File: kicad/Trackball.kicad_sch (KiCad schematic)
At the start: 38 parts, among them J1 Conn_01x04, J101 Conn_02x03_Counter_Clockwise, SW1 Push_Button, SW101 Push_Button, SW102 Push_Button, SW103 Push_Button, SW104 Push_Button, SW106 Push_Button, SW2 Push_Button, SW3 RotaryEncoder_Switch_MP, U103 TCR2EF19, U2 PMW3360, U4 TLV73333PDBV, U7 ESP32-S3-WROOM-2

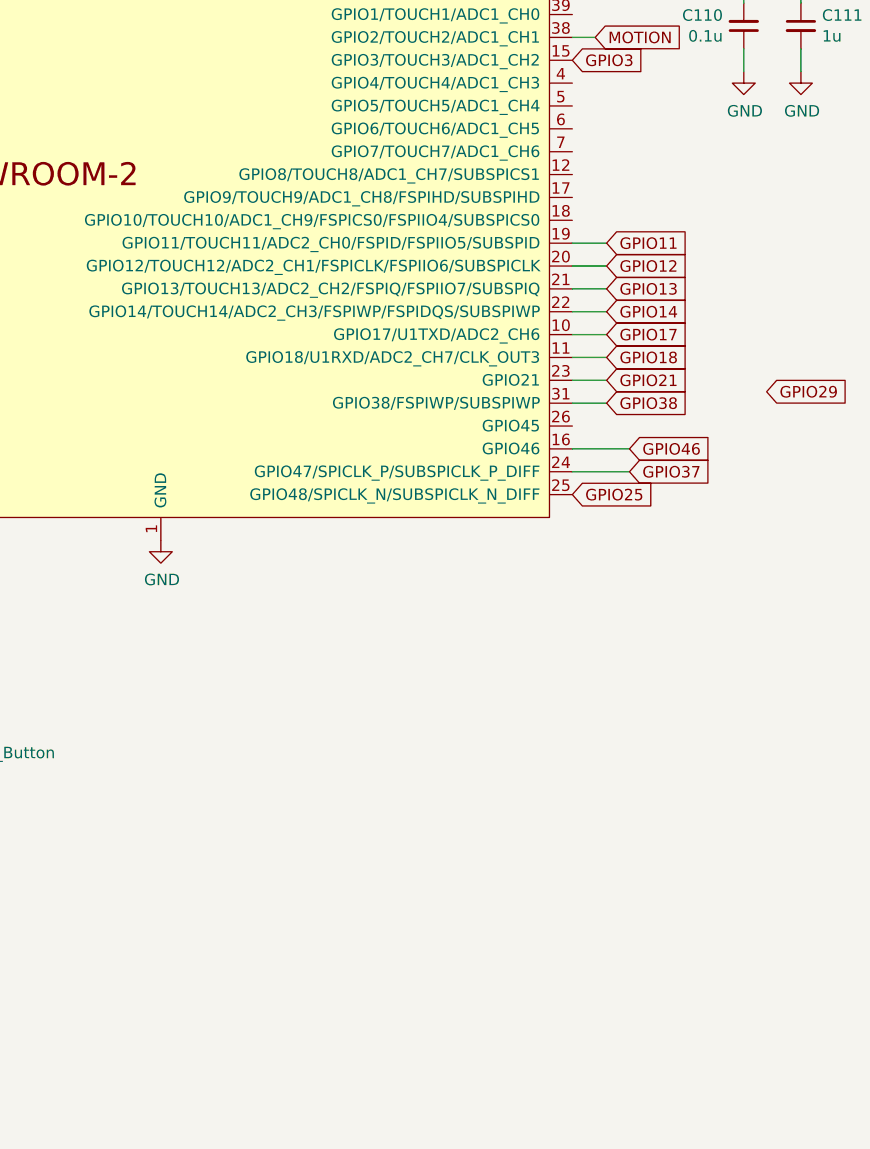
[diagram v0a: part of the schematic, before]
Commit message: V1 prebuild
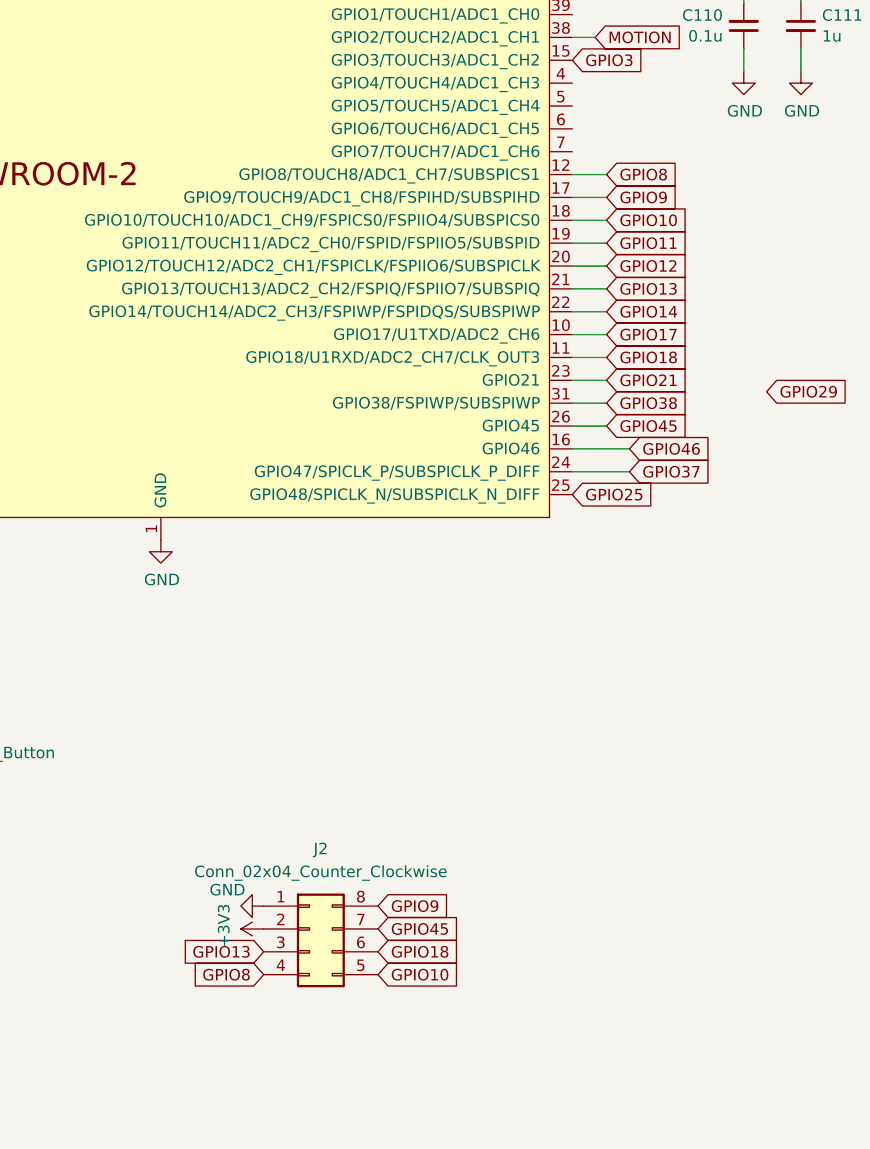
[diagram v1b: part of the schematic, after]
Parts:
- added J2: Conn_02x04_Counter_Clockwise, Connector_IDC:IDC-Header_2x04_P2.54mm_Vertical, symbol Connector_Generic:Conn_02x04_Counter_Clockwise
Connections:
- net +3V3: now also J2.2 (Pin_2)
- net GND: now also J2.1 (Pin_1)
- net GPIO13: now also J2.3 (Pin_3)
- net GPIO18: now also J2.6 (Pin_6)
- net GPIO8: now reaches U7.12 (GPIO8/TOUCH8/ADC1_CH7/SUBSPICS1)
- net GPIO8: now also J2.4 (Pin_4)
- net GPIO9: now reaches U7.17 (GPIO9/TOUCH9/ADC1_CH8/FSPIHD/SUBSPIHD)
- net GPIO9: now also J2.8 (Pin_8)
- net GPIO10: now reaches U7.18 (GPIO10/TOUCH10/ADC1_CH9/FSPICS0/FSPIIO4/SUBSPICS0)
- net GPIO10: now also J2.5 (Pin_5)
- net GPIO45: now reaches U7.26 (GPIO45)
- net GPIO45: now also J2.7 (Pin_7)
